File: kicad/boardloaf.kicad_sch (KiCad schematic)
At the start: 43 parts, among them J1 AudioJack4, J2 AudioJack4, SW1 SW_Push, SW10 SW_Push, SW11 SW_Push, SW12 SW_Push, SW13 SW_Push, SW14 SW_Push, SW15 SW_Push, SW16 SW_Push, SW17 SW_Push, SW18 SW_Push, SW2 SW_Push, SW3 SW_Push, SW4 SW_Push, SW5 SW_Push, SW6 SW_Push, SW7 SW_Push, SW8 SW_Push, SW9 SW_Push, U1 RP2040-Zero

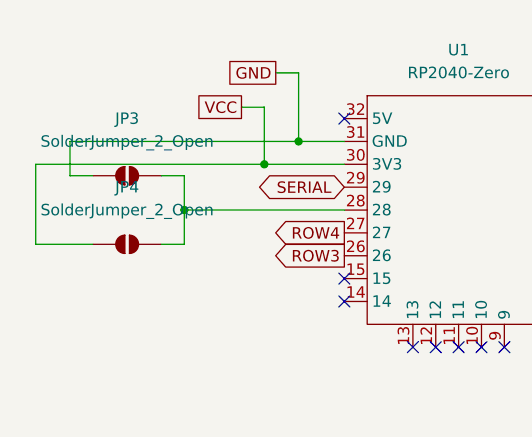
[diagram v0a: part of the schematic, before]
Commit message: Update boardloaf.kicad_sch
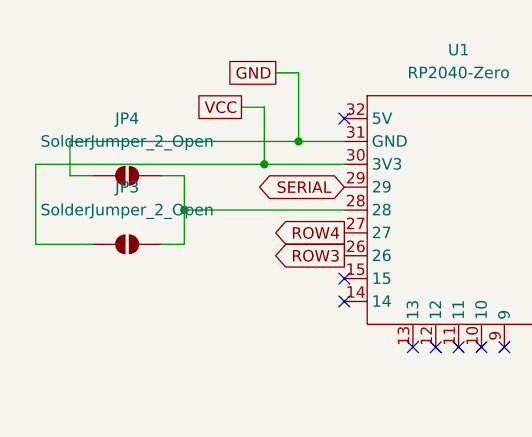
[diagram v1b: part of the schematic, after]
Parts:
- renumbered JP4 to JP3, JP3 to JP4
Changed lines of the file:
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@@
 		(dnp no)
 		(fields_autoplaced yes)
-		(property "Reference" "JP4"
+		(property "Reference" "JP3"
 			(at 29.21 35.56 0)
 			(effects
@@
 			(project "boardloaf"
 				(path "/3a093344-253b-4353-a388-64989d9a245c"
-					(reference "JP4")
+					(reference "JP3")
 					(unit 1)
 				)
@@
 		(dnp no)
 		(fields_autoplaced yes)
-		(property "Reference" "JP3"
+		(property "Reference" "JP4"
 			(at 29.21 27.94 0)
 			(effects
@@
 			(project "boardloaf"
 				(path "/3a093344-253b-4353-a388-64989d9a245c"
-					(reference "JP3")
+					(reference "JP4")
 					(unit 1)
 				)
